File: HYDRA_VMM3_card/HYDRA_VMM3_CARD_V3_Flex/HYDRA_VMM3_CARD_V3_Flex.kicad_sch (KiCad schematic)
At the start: 24 parts, among them J1 ME1014010101011, J2 FPC: 68711714522, J3 FPC_4pin

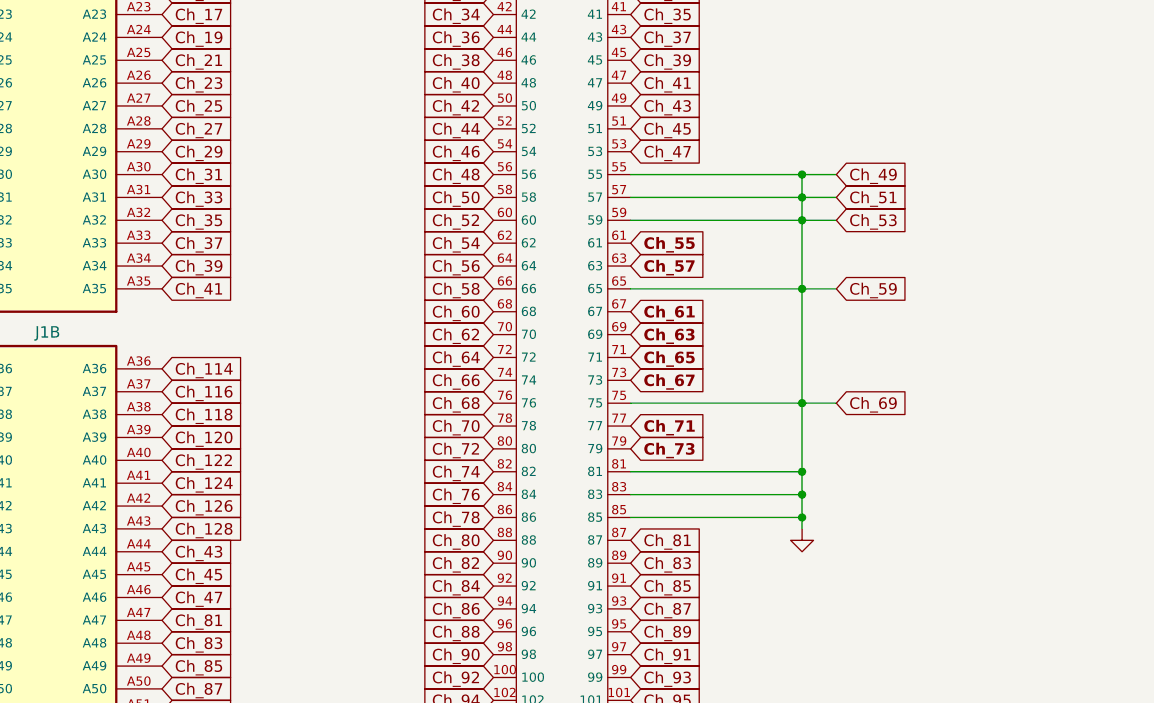
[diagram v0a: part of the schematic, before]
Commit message: .
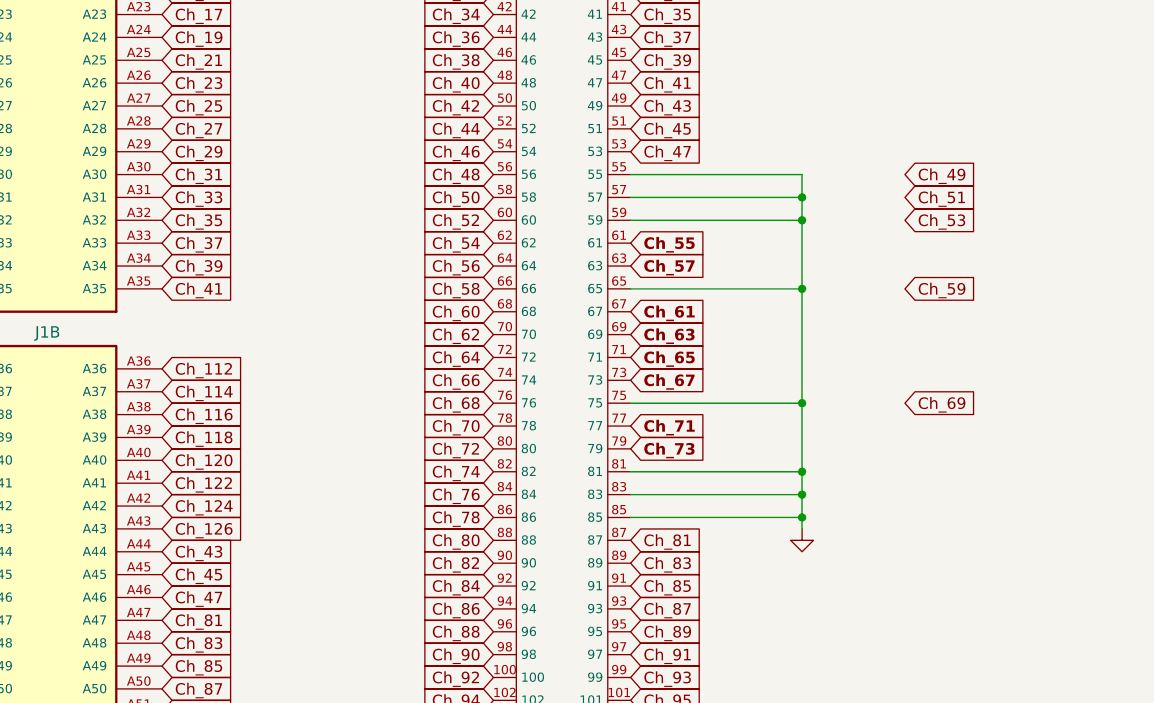
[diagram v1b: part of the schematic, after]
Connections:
- net Ch_128 is gone; now on net Ch_126: J1.A43
- net Ch_112: now also J1.A36
- net Ch_114: now also J1.A37; no longer J1.A36
- net Ch_116: now also J1.A38; no longer J1.A37
- net Ch_118: now also J1.A39; no longer J1.A38
- net Ch_120: now also J1.A40; no longer J1.A39
- net Ch_122: now also J1.A41; no longer J1.A40
- net Ch_124: now also J1.A42; no longer J1.A41
- net Ch_126: no longer J1.A42
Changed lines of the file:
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@@
 	)
 	(junction
-		(at 172.72 134.62)
-		(diameter 0)
-		(color 0 0 0 0)
-	)
-	(junction
 		(at 73.66 60.96)
 		(diameter 0)
@@
 	(wire
 		(pts
-			(xy 172.72 134.62) (xy 176.53 134.62)
-		)
-		(stroke
-			(width 0)
-			(type default)
-		)
-	)
-	(wire
-		(pts
 			(xy 172.72 139.7) (xy 172.72 147.32)
 		)
@@
 	(wire
 		(pts
-			(xy 172.72 137.16) (xy 176.53 137.16)
-		)
-		(stroke
-			(width 0)
-			(type default)
-		)
-	)
-	(wire
-		(pts
 			(xy 172.72 173.99) (xy 172.72 172.72)
 		)
@@
 	(wire
 		(pts
-			(xy 172.72 139.7) (xy 176.53 139.7)
-		)
-		(stroke
-			(width 0)
-			(type default)
-		)
-	)
-	(wire
-		(pts
 			(xy 73.66 60.96) (xy 72.39 60.96)
 		)
@@
 	(wire
 		(pts
-			(xy 172.72 160.02) (xy 176.53 160.02)
-		)
-		(stroke
-			(width 0)
-			(type default)
-		)
-	)
-	(wire
-		(pts
 			(xy 111.76 41.91) (xy 111.76 44.45)
 		)
@@
 	(wire
 		(pts
-			(xy 172.72 147.32) (xy 176.53 147.32)
-		)
-		(stroke
-			(width 0)
-			(type default)
-		)
-	)
-	(wire
-		(pts
 			(xy 297.18 101.6) (xy 285.75 101.6)
 		)
@@
 		)
 	)
-	(global_label "Ch_118"
+	(global_label "Ch_116"
 		(shape input)
 		(at 101.6 161.29 0)
@@
 		)
 	)
-	(global_label "Ch_120"
+	(global_label "Ch_118"
 		(shape input)
 		(at 101.6 163.83 0)
@@
 	(global_label "Ch_53"
 		(shape input)
-		(at 176.53 139.7 0)
+		(at 184.15 139.7 0)
 		(fields_autoplaced yes)
 		(effects
@@
 		)
 		(property "Intersheetrefs" "${INTERSHEET_REFS}"
-			(at 185.3208 139.7 0)
+			(at 192.9408 139.7 0)
 			(effects
 				(font
@@
 	(global_label "Ch_49"
 		(shape input)
-		(at 176.53 134.62 0)
+		(at 184.15 134.62 0)
 		(fields_autoplaced yes)
 		(effects
@@
 		)
 		(property "Intersheetrefs" "${INTERSHEET_REFS}"
-			(at 185.3208 134.62 0)
+			(at 192.9408 134.62 0)
 			(effects
 				(font
@@
 	(global_label "Ch_51"
 		(shape input)
-		(at 176.53 137.16 0)
+		(at 184.15 137.16 0)
 		(fields_autoplaced yes)
 		(effects
@@
 		)
 		(property "Intersheetrefs" "${INTERSHEET_REFS}"
-			(at 185.3208 137.16 0)
+			(at 192.9408 137.16 0)
 			(effects
 				(font
@@
 		)
 	)
-	(global_label "Ch_128"
+	(global_label "Ch_126"
 		(shape input)
 		(at 101.6 173.99 0)
@@
 		)
 	)
-	(global_label "Ch_114"
+	(global_label "Ch_112"
 		(shape input)
 		(at 101.6 156.21 0)
@@
 		)
 	)
-	(global_label "Ch_116"
+	(global_label "Ch_114"
 		(shape input)
 		(at 101.6 158.75 0)
@@
 	(global_label "Ch_69"
 		(shape input)
-		(at 176.53 160.02 0)
+		(at 184.15 160.02 0)
 		(fields_autoplaced yes)
 		(effects
@@
 		)
 		(property "Intersheetrefs" "${INTERSHEET_REFS}"
-			(at 185.3208 160.02 0)
+			(at 192.9408 160.02 0)
 			(effects
 				(font
@@
 		)
 	)
-	(global_label "Ch_126"
+	(global_label "Ch_124"
 		(shape input)
 		(at 101.6 171.45 0)
@@
 		)
 	)
-	(global_label "Ch_122"
+	(global_label "Ch_120"
 		(shape input)
 		(at 101.6 166.37 0)
@@
 	(global_label "Ch_59"
 		(shape input)
-		(at 176.53 147.32 0)
+		(at 184.15 147.32 0)
 		(fields_autoplaced yes)
 		(effects
@@
 		)
 		(property "Intersheetrefs" "${INTERSHEET_REFS}"
-			(at 185.3208 147.32 0)
+			(at 192.9408 147.32 0)
 			(effects
 				(font
@@
 		)
 	)
-	(global_label "Ch_124"
+	(global_label "Ch_122"
 		(shape input)
 		(at 101.6 168.91 0)
